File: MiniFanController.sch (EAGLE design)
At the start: 23 parts, among them J1 MOLEX_47053-1000MOLEX_47053-1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, J2 MOLEX_47053-1000MOLEX_47053-1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, J3 MOLEX_47053-1000MOLEX_47053-1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, J5 TSW-102-07-G-S, Q1 MICRO_COMMERCIAL_MMSS8050-L-T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, Q2 DIODES_INC_DMP3099L-13DIODES_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, Q3 MICRO_COMMERCIAL_MMSS8050-L-T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, Q4 MICRO_COMMERCIAL_MMSS8050-L-T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, Q5 DIODES_INC_DMP3099L-13DIODES_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, Q6 MICRO_COMMERCIAL_MMSS8050-L-T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, U1 NANO_FOOTPRINT

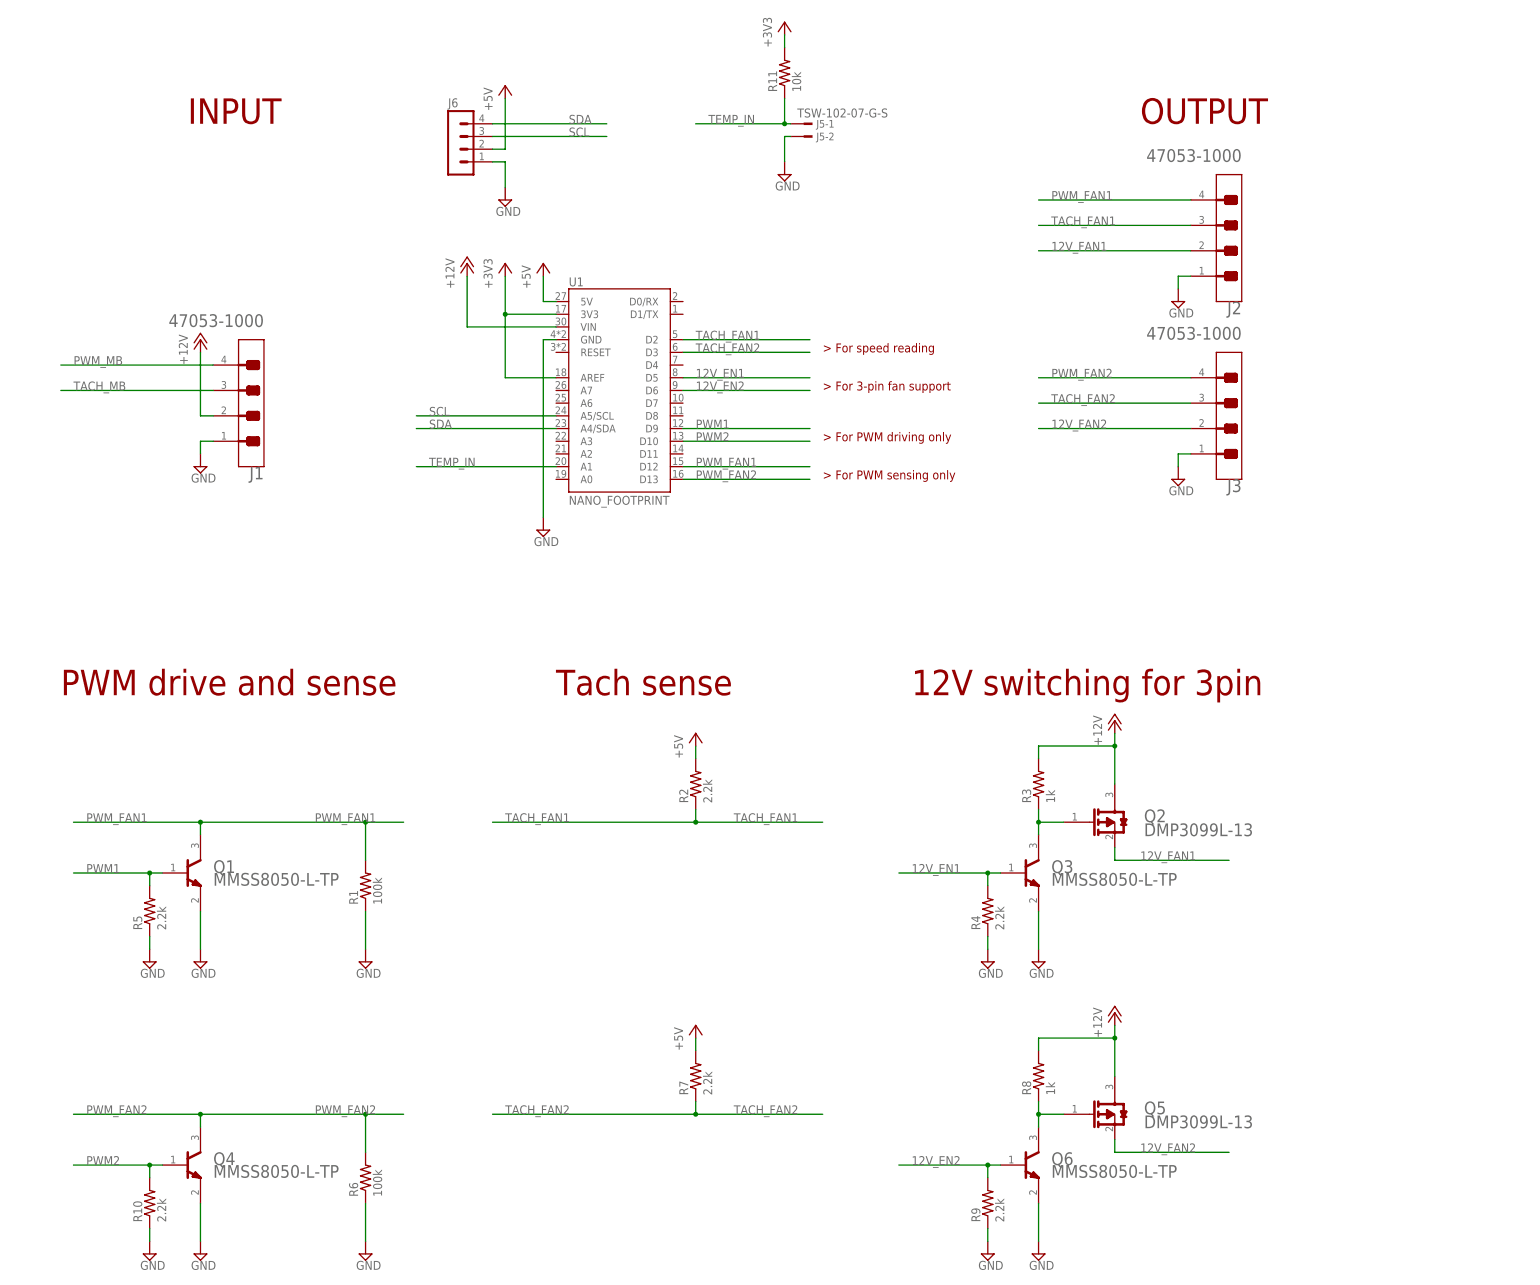
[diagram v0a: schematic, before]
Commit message: v2 commit. Added current limiting base resistors (oops)
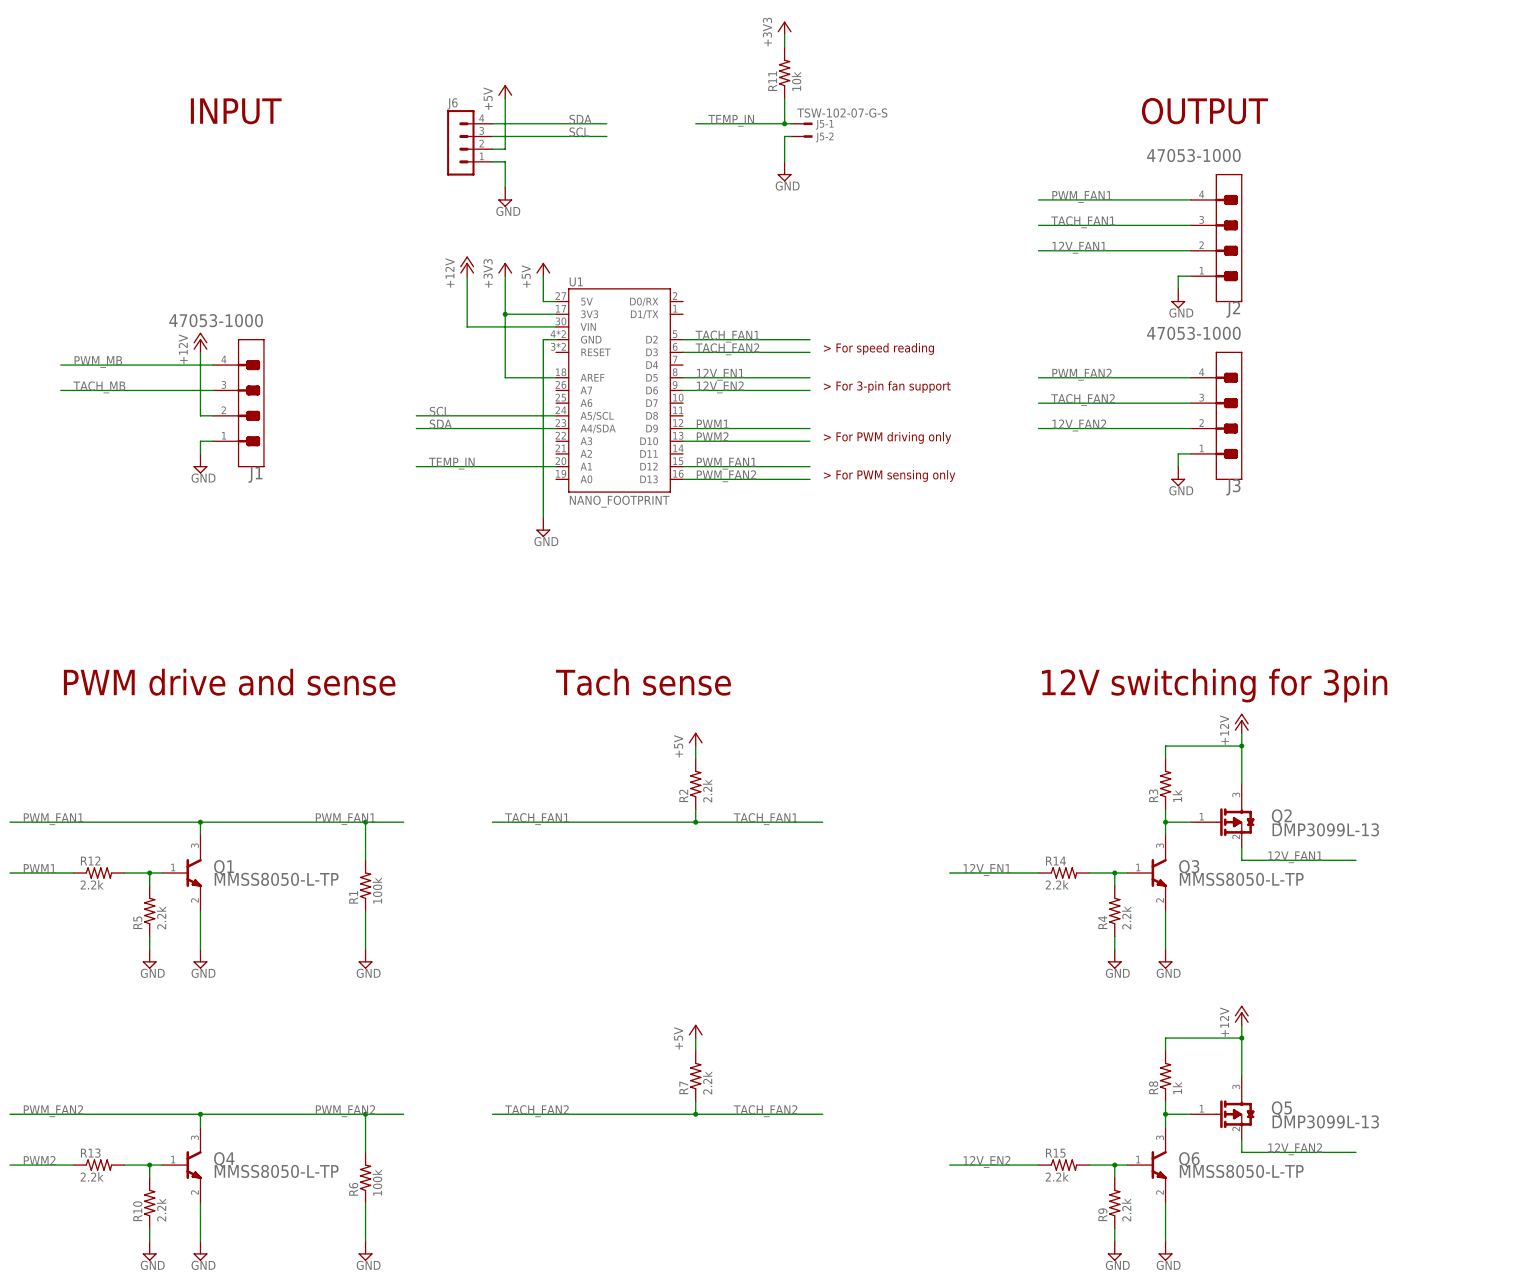
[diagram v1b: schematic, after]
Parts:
- added R12, R13, R14, R15: 2.2k, rcl:R-US_R0603
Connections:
- new net N$3: Q1.B, R12.2, R5.2
- new net N$4: Q4.B, R10.2, R13.2
- new net N$5: Q3.B, R14.2, R4.2
- new net N$6: Q6.B, R15.2, R9.2
- net 12V_EN1: now also R14.1; no longer Q3.B, R4.2
- net 12V_EN2: now also R15.1; no longer Q6.B, R9.2
- net PWM1: now also R12.1; no longer Q1.B, R5.2
- net PWM2: now also R13.1; no longer Q4.B, R10.2
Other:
- moved on the sheet: Q2, Q3, Q5, Q6, R3, R4, R8, R9
